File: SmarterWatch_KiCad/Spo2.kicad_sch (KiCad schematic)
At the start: 7 parts, among them U10 MAX30102, U9 MIC5365-1.8YC5

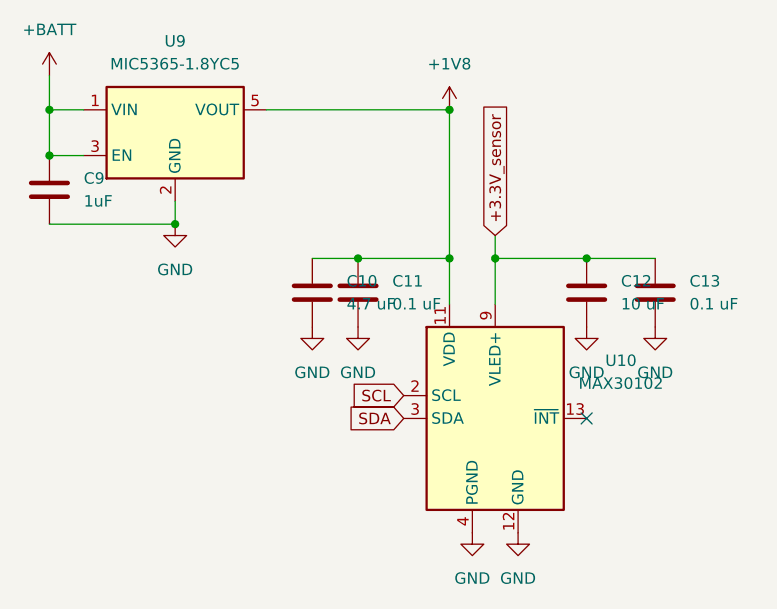
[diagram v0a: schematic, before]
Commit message: order
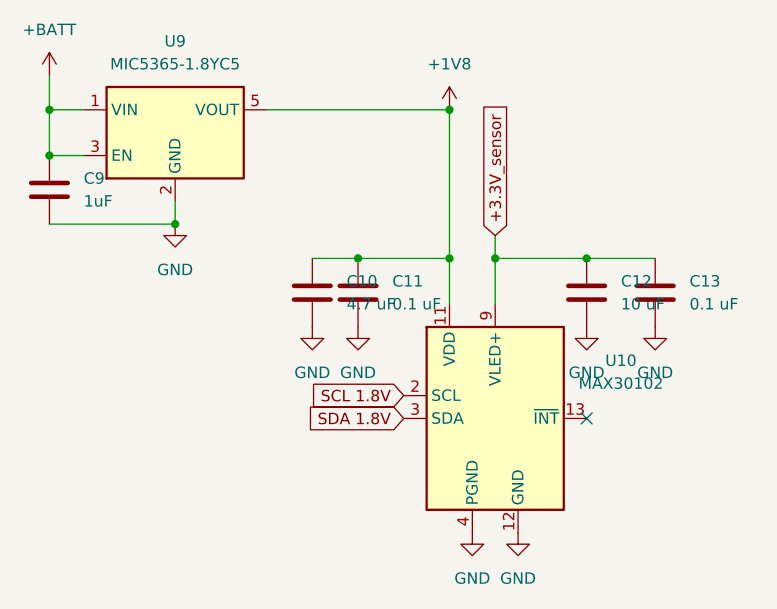
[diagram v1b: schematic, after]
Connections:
- net SCL renamed SCL 1.8V
- net SDA renamed SDA 1.8V
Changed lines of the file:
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@@
 		)
 	)
-	(global_label "SDA"
+	(global_label "SDA 1.8V"
 		(shape input)
 		(at 124.46 96.52 180)
@@
 		)
 		(property "Intersheetrefs" "${INTERSHEET_REFS}"
-			(at 117.9067 96.52 0)
+			(at 112.8267 96.52 0)
 			(effects
 				(font
@@
 		)
 	)
-	(global_label "SCL"
+	(global_label "SCL 1.8V"
 		(shape input)
 		(at 124.46 93.98 180)
@@
 		)
 		(property "Intersheetrefs" "${INTERSHEET_REFS}"
-			(at 117.9672 93.98 0)
+			(at 112.8872 93.98 0)
 			(effects
 				(font

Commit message: Footprint Stuff
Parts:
- U10: footprint OptoDevice:Maxim_OLGA-14_3.3x5.6mm_P0.8mm -> (none)
- U9: footprint Package_TO_SOT_SMD:SOT-353_SC-70-5 -> (none)
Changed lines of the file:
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@@
 			)
 		)
-		(property "Footprint" "Package_TO_SOT_SMD:SOT-353_SC-70-5"
+		(property "Footprint" ""
 			(at 99.06 53.34 0)
 			(effects
@@
 			)
 		)
-		(property "Footprint" "OptoDevice:Maxim_OLGA-14_3.3x5.6mm_P0.8mm"
+		(property "Footprint" ""
 			(at 134.62 99.06 0)
 			(effects

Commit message: Foot
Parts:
- U9: footprint (none) -> Custom_Foot:SOT65P210X110-5N
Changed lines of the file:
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@@
 			)
 		)
-		(property "Footprint" ""
+		(property "Footprint" "Custom_Foot:SOT65P210X110-5N"
 			(at 99.06 53.34 0)
 			(effects

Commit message: footprint
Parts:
- U10: footprint (none) -> Custom_Foot:XDCR_MAX30101EFD_
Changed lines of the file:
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@@
 			)
 		)
-		(property "Footprint" ""
+		(property "Footprint" "Custom_Foot:XDCR_MAX30101EFD_"
 			(at 134.62 99.06 0)
 			(effects

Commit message: added pad to symbol
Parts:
- U10: footprint Custom_Foot:XDCR_MAX30101EFD_ -> (none)
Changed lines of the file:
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@@
 			)
 		)
-		(property "Footprint" "Custom_Foot:XDCR_MAX30101EFD_"
+		(property "Footprint" ""
 			(at 134.62 99.06 0)
 			(effects
